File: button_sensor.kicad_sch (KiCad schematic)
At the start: 46 parts, among them J21 Conn_01x10, J22 Conn_01x10, U2 74HC138, U26 LTV-817S, U27 LTV-817S, U34 LTV-817S, U35 LTV-817S, U36 LTV-817S, U37 LTV-817S, U38 LTV-817S, U39 LTV-817S

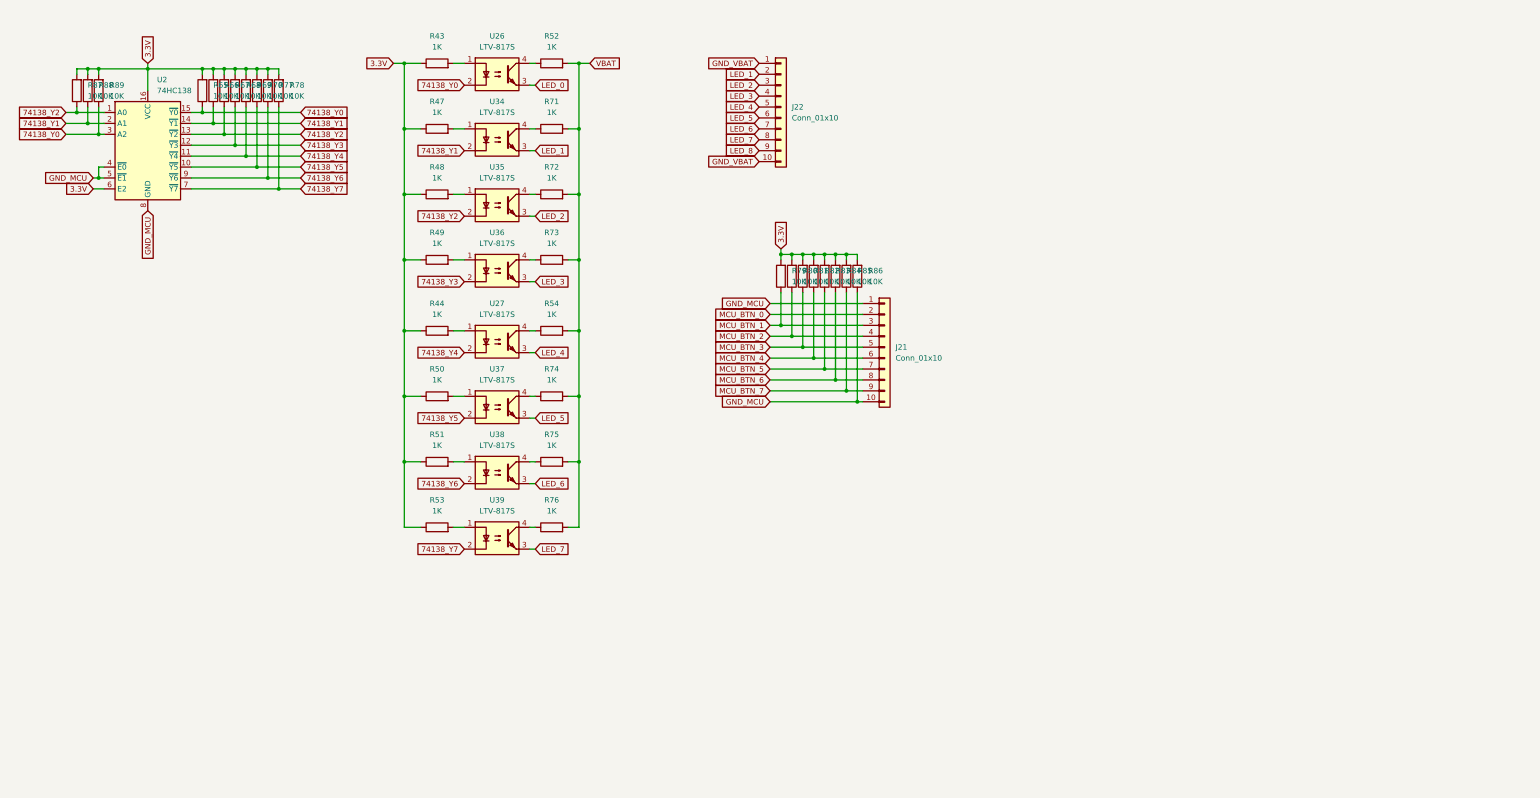
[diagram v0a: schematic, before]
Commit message: new file:   decon_ctrl.pdf
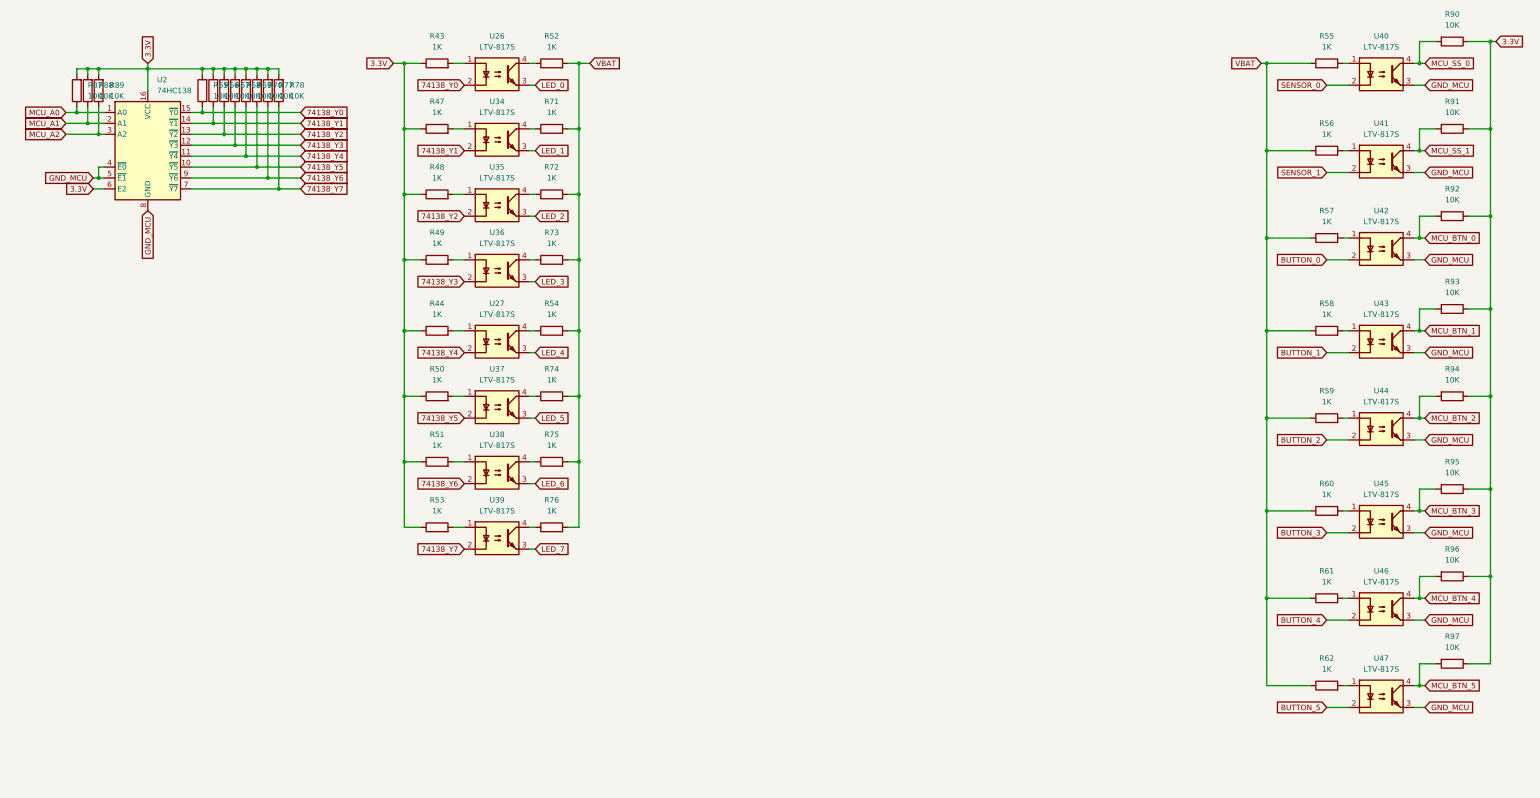
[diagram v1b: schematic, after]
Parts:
- removed J21, J22: Conn_01x10, Connector_Phoenix_MC:PhoenixContact_MC_1,5_10-G-3.81_1x10_P3.81mm_Horizontal, symbol Connector_Generic:Conn_01x10
- removed R79, R80, R81, R82, R83, R84, R85, R86: 10K, Resistor_SMD:R_0805_2012Metric, symbol Device:R
- added R55, R56, R57, R58, R59, R60, R61, R62: 1K, Resistor_SMD:R_0805_2012Metric, symbol Device:R
- added R90, R91, R92, R93, R94, R95, R96, R97: 10K, Resistor_SMD:R_0805_2012Metric, symbol Device:R
- added U40, U41, U42, U43, U44, U45, U46, U47: LTV-817S, Package_DIP:SMDIP-4_W9.53mm, symbol Isolator:LTV-817S
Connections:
- net 3.3V: now also R90.1, R91.1, R92.1, R93.1, R94.1, R95.1, R96.1, R97.1
- net 74138_Y0: no longer R89.1, U2.3 (A2)
- net 74138_Y1: no longer R88.1, U2.2 (A1)
- net 74138_Y2: no longer R87.1, U2.1 (A0)
- net GND_MCU: now also U40.3, U41.3, U42.3, U43.3, U44.3, U45.3, U46.3, U47.3
- net MCU_BTN_0: now also R92.2, U42.4
- net MCU_BTN_1: now also R93.2, U43.4
- net MCU_BTN_2: now also R94.2, U44.4
- net MCU_BTN_3: now also R95.2, U45.4
- net MCU_BTN_4: now also R96.2, U46.4
- net MCU_BTN_5: now also R97.2, U47.4
- net VBAT: now also R55.1, R56.1, R57.1, R58.1, R59.1, R60.1, R61.1, R62.1
- new net: R59.2, U44.1
- new net: R61.2, U46.1
- new net: R62.2, U47.1
- new net: R55.2, U40.1
- new net: R57.2, U42.1
- new net: R58.2, U43.1
- new net: R60.2, U45.1
- new net: R56.2, U41.1
- new net BUTTON_0: U42.2
- new net BUTTON_1: U43.2
- new net BUTTON_2: U44.2
- new net BUTTON_3: U45.2
- new net BUTTON_4: U46.2
- new net BUTTON_5: U47.2
- new net MCU_A0: R87.1, U2.1 (A0)
- new net MCU_A1: R88.1, U2.2 (A1)
- new net MCU_A2: R89.1, U2.3 (A2)
- new net MCU_SS_0: R90.2, U40.4
- new net MCU_SS_1: R91.2, U41.4
- new net SENSOR_0: U40.2
- new net SENSOR_1: U41.2

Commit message: modified:   DECON_Ctrl_Panel.kicad_pcb
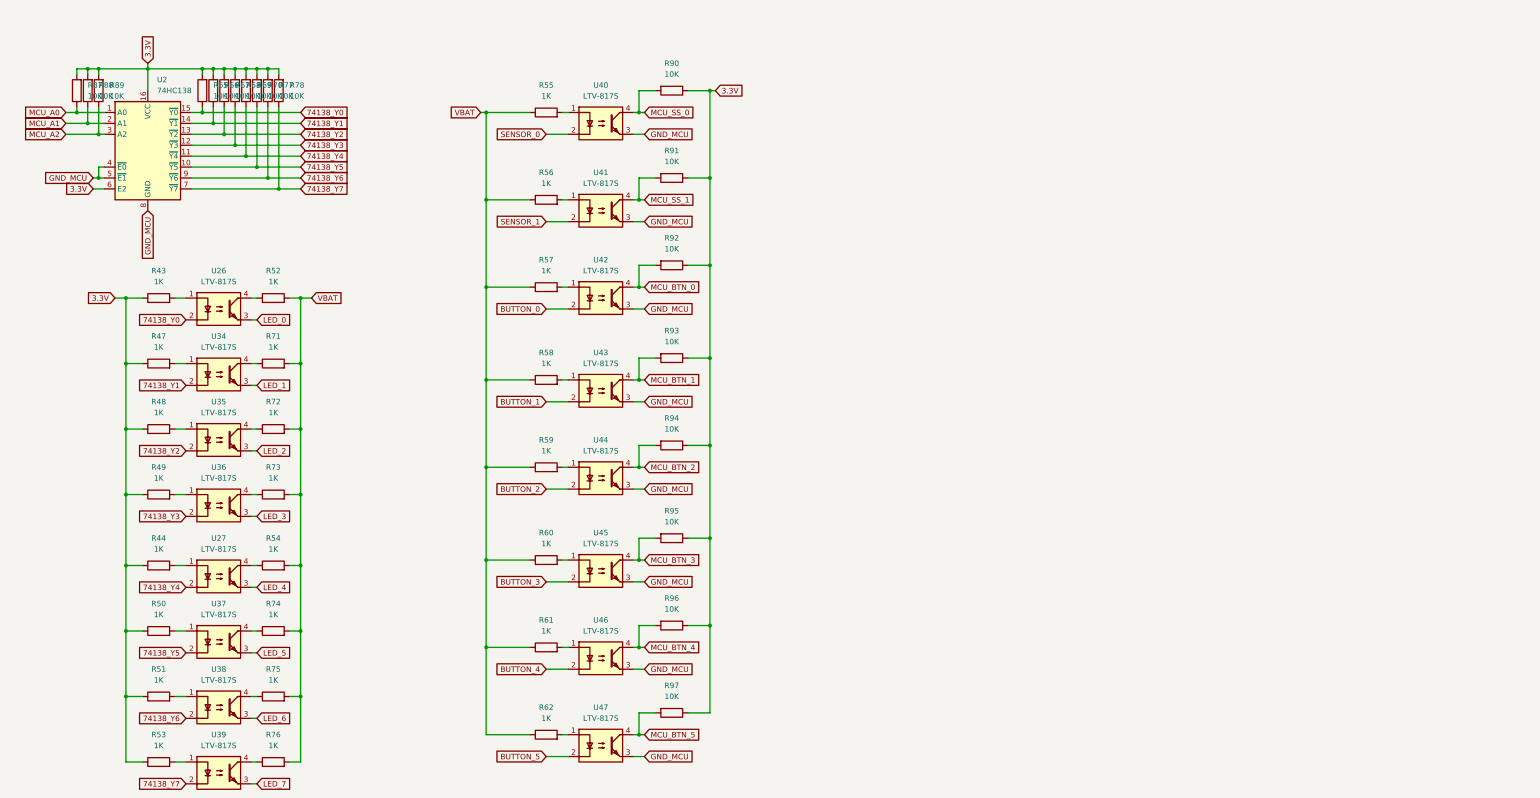
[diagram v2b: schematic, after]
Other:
- moved on the sheet: R43, R44, R47, R48, R49, R50, R51, R52, R53, R54, R55, R56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
